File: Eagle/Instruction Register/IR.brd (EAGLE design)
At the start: 160 x 100 mm, 55 parts, among them IC1 SN74HC04N, IC2 SN74HC04N, J1 55959-2030, J2 55959-2430

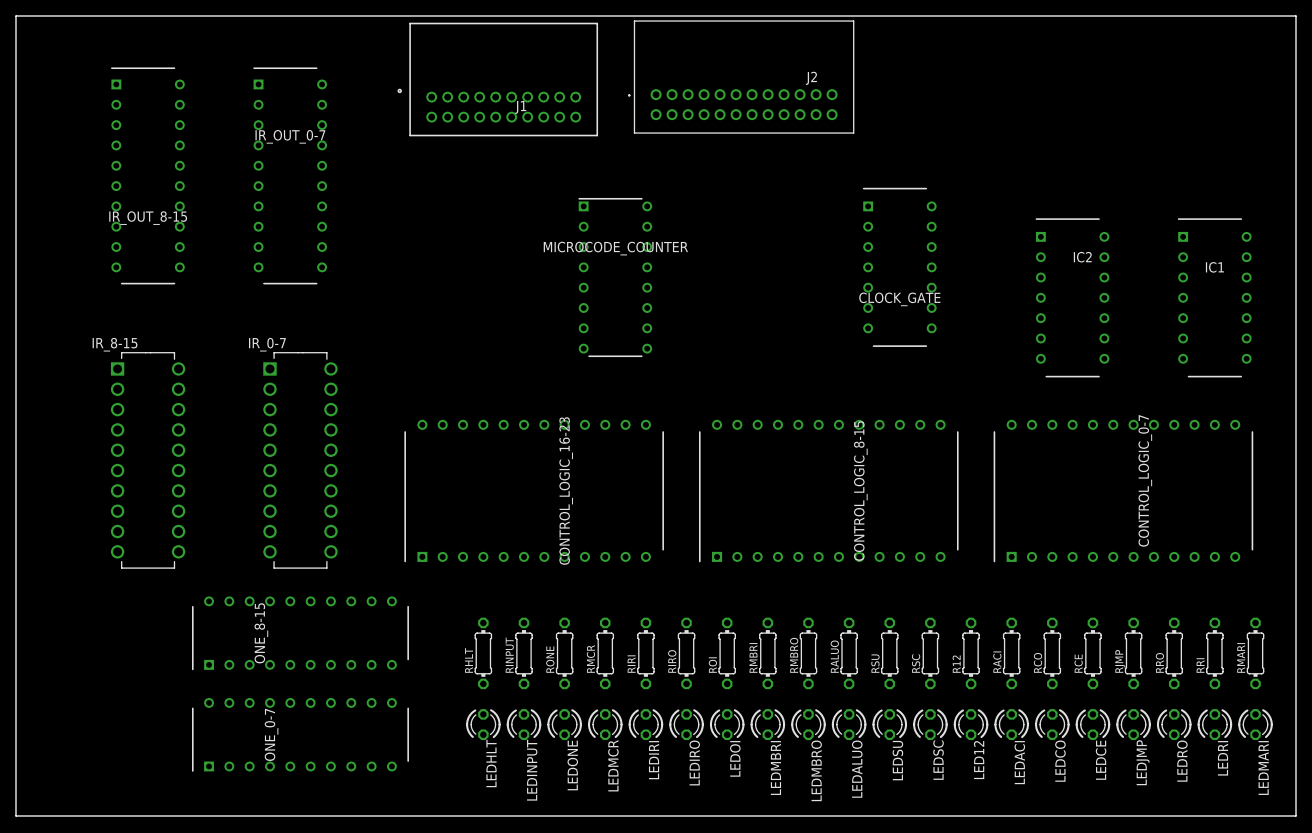
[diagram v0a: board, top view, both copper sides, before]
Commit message: finished most boards
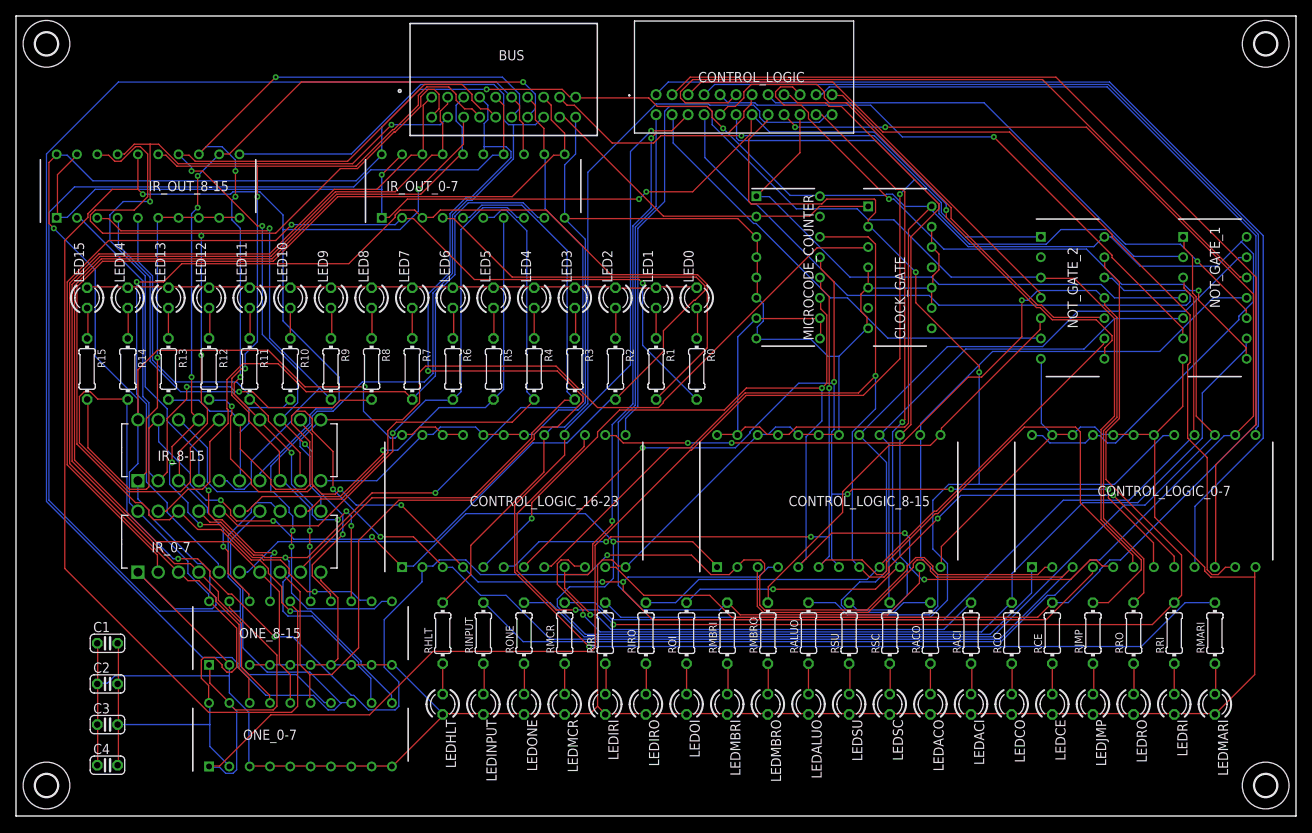
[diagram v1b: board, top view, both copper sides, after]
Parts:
- added C1, C2, C3, C4: (no value), rcl:C025-024X044
- added LED0, LED1, LED10, LED11, LED2, LED3, LED4, LED5, LED6, LED7, LED8, LED9: YELLOW, led:LED3MM
- added LED13, LED14, LED15, LEDACO: BLUE, led:LED3MM
- added R0, R1, R10, R11, R13, R14, R15, R2, R3, R4, R5, R6, R7, R8, R9, RACO: 220, rcl:0204/7
- added U$1, U$2, U$3, U$4: (no value), holes:2,8
- moved LED12 109.2 mm to (24.1, 64.8), turned to 90 degrees
- moved R12 101.7 mm to (24.1, 55.9), turned to 270 degrees
- moved IR_8-15 24.3 mm to (38.1, 49.5), turned to 90 degrees
- moved IR_OUT_0-7 22.9 mm to (57.1, 78.7), turned to 90 degrees
- moved MICROCODE_COUNTER 21.6 mm to (96.5, 68.6)
- moved LEDCE 5.68 mm to (129.5, 14.0)
- moved LEDOI 5.68 mm to (83.8, 14.0)
- moved LEDRI 5.68 mm to (144.8, 14.0)
- moved LEDRO 5.68 mm to (139.7, 14.0)
- moved RCE 5.68 mm to (129.5, 22.9)
- moved ROI 5.68 mm to (83.8, 22.9)
- moved RRI 5.68 mm to (144.8, 22.9)
- moved RRO 5.68 mm to (139.7, 22.9)
- moved LEDACI 5.68 mm to (119.4, 14.0)
- moved LEDALUO 5.68 mm to (99.1, 14.0)
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- renumbered IC1 to NOT_GATE_1, IC2 to NOT_GATE_2, J1 to BUS, J2 to CONTROL_LOGIC
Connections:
- new net N$21: LEDACO.A, RACO.1
- new net N$25: LED1.A, R1.1
- new net N$26: LED2.A, R2.1
- new net N$27: LED3.A, R3.1
- new net N$28: LED4.A, R4.1
- new net N$29: LED5.A, R5.1
- new net N$30: LED6.A, R6.1
- new net N$31: LED7.A, R7.1
- new net N$32: LED8.A, R8.1
- new net N$34: LED9.A, R9.1
- new net N$35: LED10.A, R10.1
- new net N$36: LED11.A, R11.1
- new net N$38: LED13.A, R13.1
- new net N$39: LED14.A, R14.1
- new net N$40: LED15.A, R15.1
- new net N$41: LED0.A, R0.1
- new net N$42: LED0.K, LED1.K, LED10.K, LED11.K, LED12.K, LED13.K, LED14.K, LED15.K, LED2.K, LED3.K, LED4.K, LED5.K, LED6.K, LED7.K, LED8.K, LED9.K
- net ACO: now also RACO.2; no longer R12.2
- net GND: now also C1.1, C2.1, C3.1, C4.1, LEDACO.K; no longer LED12.K
- net IR0: now also R0.2
- net IR1: now also R1.2
- net IR10: now also R10.2
- net IR11: now also R11.2
- net IR12: now also R12.2
- net IR13: now also R13.2
- net IR14: now also R14.2
- net IR15: now also R15.2
- net IR2: now also R2.2
- net IR3: now also R3.2
- net IR4: now also R4.2
- net IR5: now also R5.2
- net IR6: now also R6.2
- net IR7: now also R7.2
- net IR8: now also R8.2
- net IR9: now also R9.2
- net VCC: now also C1.2, C2.2, C3.2, C4.2
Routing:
- net GND: track 0.00 -> 633.3 mm, vias 0 -> 1
- net VCC: track 0.00 -> 472.5 mm, vias 0 -> 4
- net !ONE: track 0.00 -> 246.0 mm, vias 0 -> 1
- net IR14: track 0.00 -> 211.5 mm, vias 0 -> 3
- net IR13: track 0.00 -> 201.1 mm, vias 0 -> 2
- net B10: track 0.00 -> 200.9 mm, vias 0 -> 2
- net B5: track 0.00 -> 197.9 mm
- net INPUT: track 0.00 -> 193.4 mm, vias 0 -> 2
- net IR15: track 0.00 -> 190.8 mm, vias 0 -> 4
- net CE: track 0.00 -> 180.7 mm
- net !IRO: track 0.00 -> 173.8 mm, vias 0 -> 4
- net B4: track 0.00 -> 172.3 mm
- net MARI: track 0.00 -> 161.3 mm, vias 0 -> 2
- net IRI: track 0.00 -> 161.3 mm, vias 0 -> 2
- net IR12: track 0.00 -> 160.3 mm, vias 0 -> 5
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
